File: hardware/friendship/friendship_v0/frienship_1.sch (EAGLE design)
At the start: 8 parts

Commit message: as far as i got tonight
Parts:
- added IC1, IC2: 74HC165D, 74xx-eu:74HC165D
- added JP1: (no value), pinhead:PINHD-2X5
- added R5: (no value), rcl:R-EU_R0603
- added T1, T2, T3, T4: BCX70SMD, transistor:BCX70SMD
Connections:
- removed net N$1: R4.2, U$4.PRSNT1
- removed net N$3: R3.2, U$2.PRSNT1
- removed net N$4: R2.2, U$1.PRSNT1
- removed net N$5: R1.2, U$3.PRSNT1
- new net PRSNT0: IC1A.A, R1.2, T1.B, U$3.PRSNT1
- new net PRSNT1: IC1A.B, R2.2, T2.B, U$1.PRSNT1
- new net PRSNT2: R3.2, T3.B, U$2.PRSNT1
- new net PRSNT3: R4.2, T4.B, U$4.PRSNT1
- net 3V3: now also JP1.1
- net GND: now also JP1.3, JP1.5, JP1.7, JP1.9
- net IRQ0: now also IC2A.A
- net IRQ1: now also IC2A.B
- net IRQ2: now also IC1A.C, IC2A.C
- net IRQ3: now also IC1A.D, IC2A.D
- net N$2: now also T1.E, T2.C
- net N$6: now also T2.E, T3.C
- net N$7: now also T3.E, T4.C
- net TCK: now also JP1.8
- net TDI: now also JP1.2, T1.C
- net TDO: now also JP1.4, T4.E
- net TMS: now also JP1.6
- net TRST: now also JP1.10
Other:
- note added: "JTAG PINOUT"
- moved on the sheet: R1, R2, R3, R4

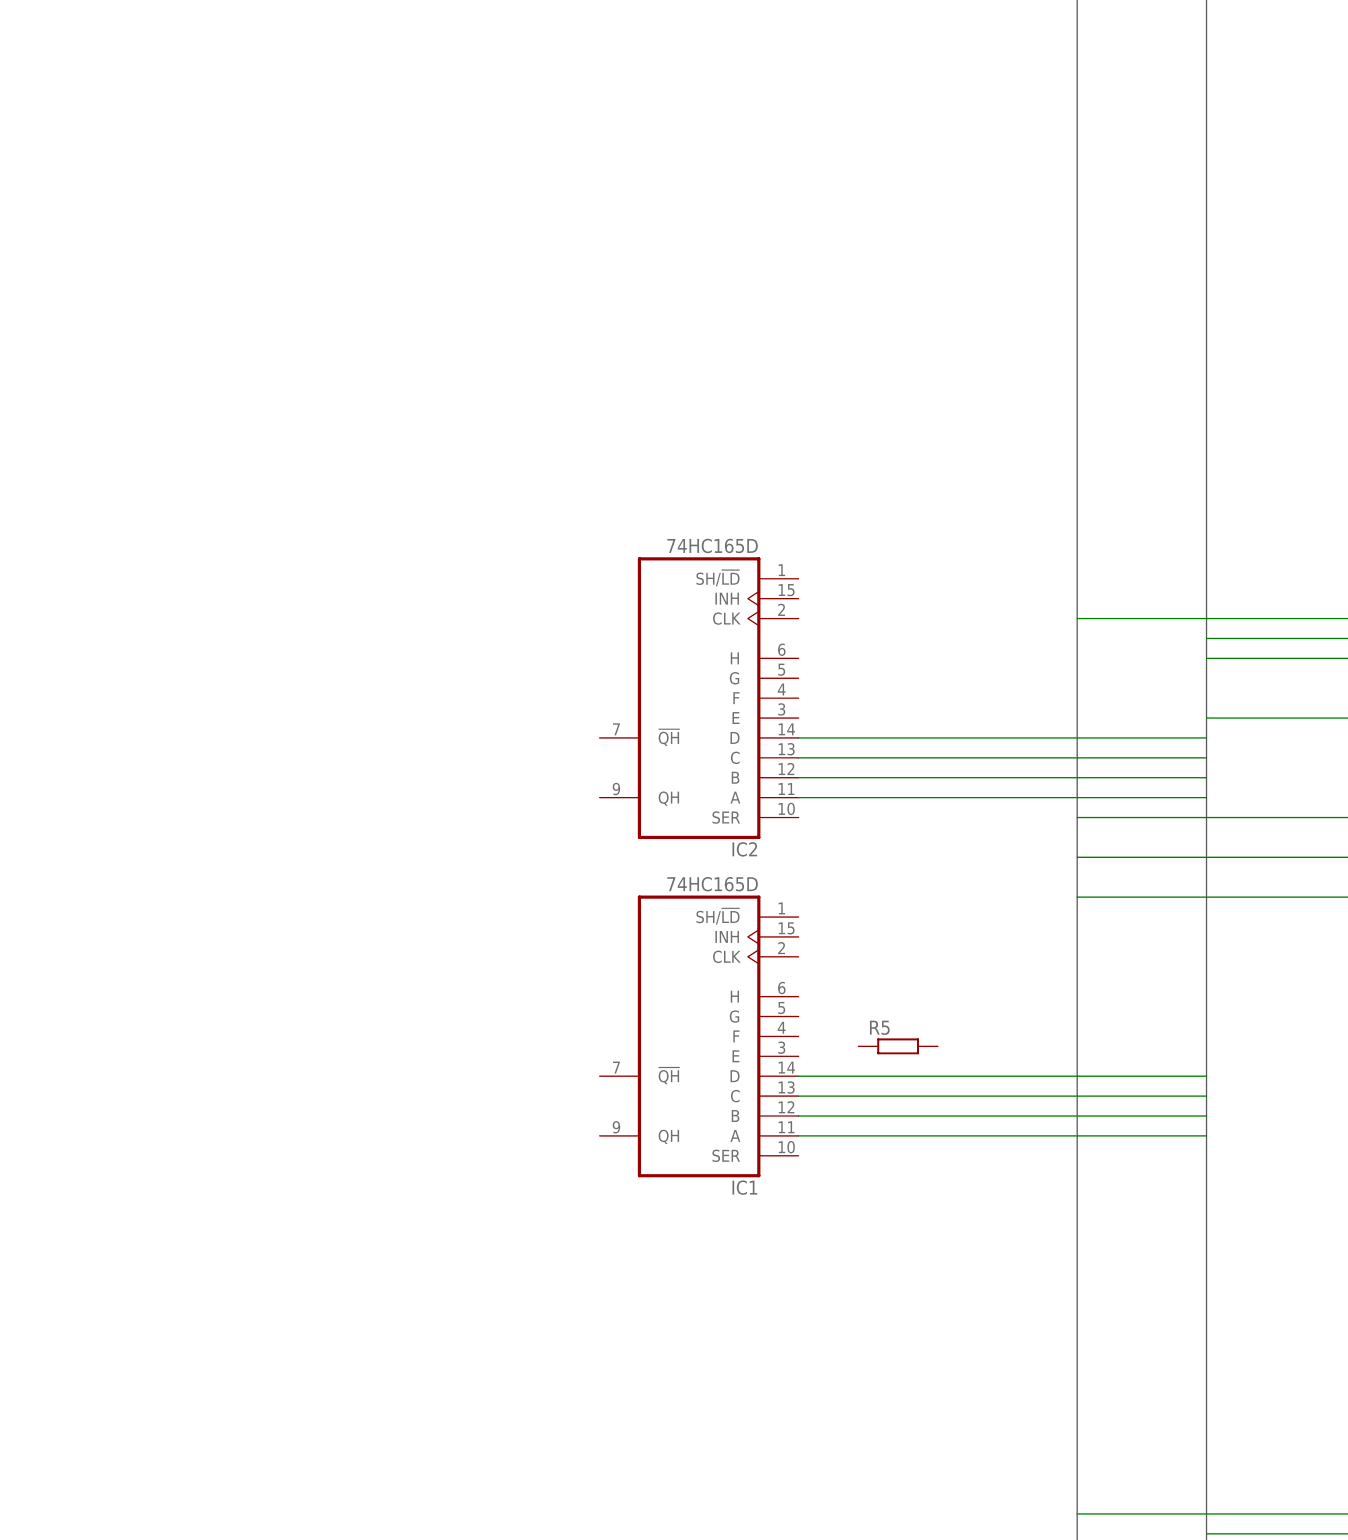
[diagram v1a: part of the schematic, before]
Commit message: initial version of friendship schematic
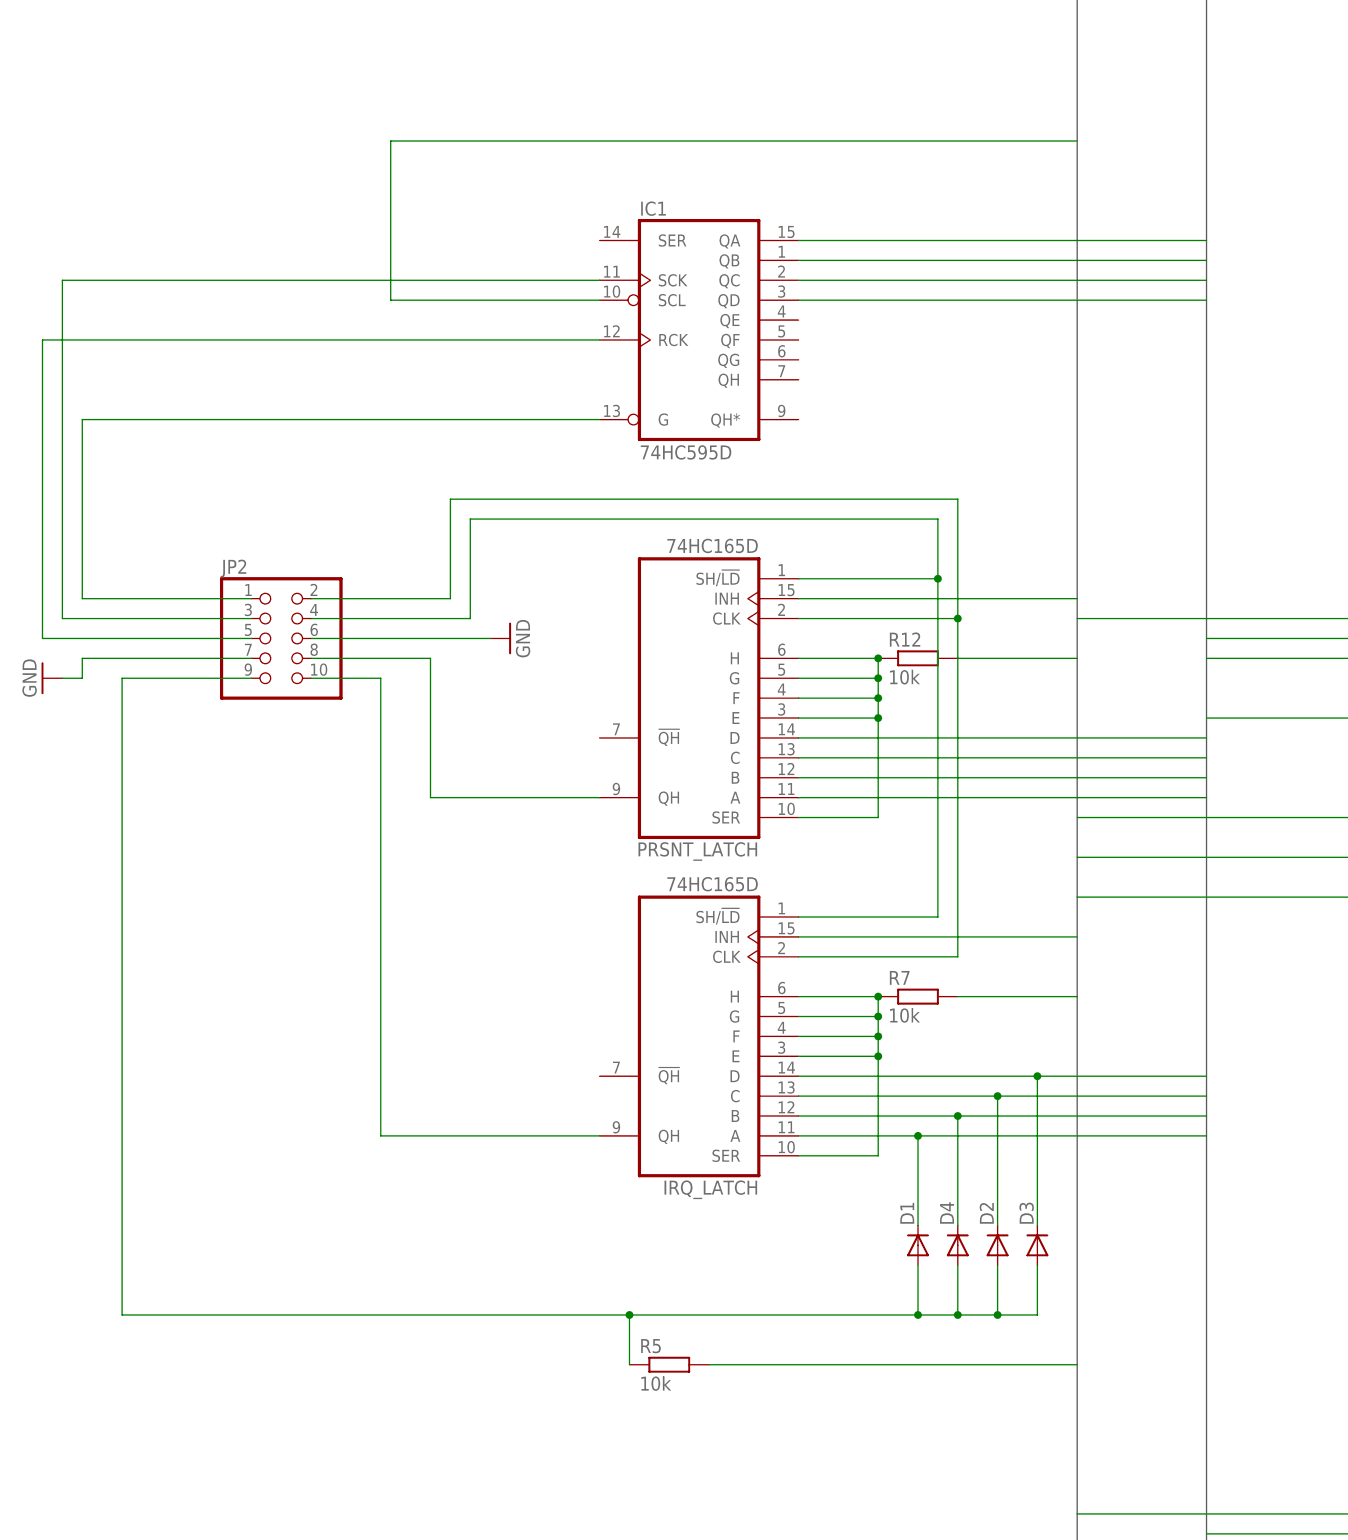
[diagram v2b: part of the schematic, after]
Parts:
- added D1, D2, D3, D4: (no value), diode:DIODE-SOD80C
- added IRQ_LATCH: 74HC165D, 74xx-eu:74HC165D
- added JP2: (no value), pinhead:PINHD-2X5
- added R12, R7: 10k, rcl:R-EU_R0603
- IC1: value 74HC165D -> 74HC595D; device 74xx-eu:74HC165D -> 74xx-eu:74HC595D
- R5: value (none) -> 10k
- renumbered IC2 to PRSNT_LATCH
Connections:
- new net N$1: IC1A.G, JP2.1
- new net N$11: D1.A, D2.A, D3.A, D4.A, JP2.9, R5.1
- new net N$13: JP2.8, PRSNT_LATCHA.QH
- new net N$17: IRQ_LATCHA.QH, JP2.10
- new net N$3: IRQ_LATCHA.SH/!LD, JP2.4, PRSNT_LATCHA.SH/!LD
- new net N$4: IC1A.SCK, JP2.3
- new net N$5: PRSNT_LATCHA.E, PRSNT_LATCHA.F, PRSNT_LATCHA.G, PRSNT_LATCHA.H, PRSNT_LATCHA.SER, R12.1
- new net N$8: IRQ_LATCHA.E, IRQ_LATCHA.F, IRQ_LATCHA.G, IRQ_LATCHA.H, IRQ_LATCHA.SER, R7.1
- new net N$9: IC1A.RCK, JP2.5
- new net SHIFT: IRQ_LATCHA.CLK, JP2.2, PRSNT_LATCHA.CLK
- net /CS0: now also IC1A.QA
- net /CS1: now also IC1A.QB
- net /CS2: now also IC1A.QC
- net /CS3: now also IC1A.QD
- net 3V3: now also IC1A.SCL, IRQ_LATCHA.INH, PRSNT_LATCHA.INH, R12.2, R5.2, R7.2
- net GND: now also JP2.6, JP2.7
- net IRQ2: now also D2.C, IRQ_LATCHA.C; no longer IC1A.C
- net IRQ3: now also D3.C, IRQ_LATCHA.D; no longer IC1A.D
- net PRSNT0: now also D1.C, IRQ_LATCHA.A; no longer IC1A.A
- net PRSNT1: now also D4.C, IRQ_LATCHA.B; no longer IC1A.B
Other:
- moved on the sheet: R5
